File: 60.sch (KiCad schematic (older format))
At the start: 183 parts, among them IC1 ATXMEGA32A4U-A, J1 USB_mini_micro_B, K1 KEYSW, K10 KEYSW, K11 KEYSW, K12 KEYSW, K13 KEYSW, K14 KEYSW, K15 KEYSW, K16 KEYSW, K17 KEYSW, K18 KEYSW, K19 KEYSW, K2 KEYSW, K20 KEYSW, K21 KEYSW, K22 KEYSW, K23 KEYSW, K24 KEYSW, K25 KEYSW, K26 KEYSW, K27 KEYSW, K28 KEYSW, K29 KEYSW, K3 KEYSW, K30 KEYSW, K31 KEYSW, K32 KEYSW, K33 KEYSW, K34 KEYSW, K35 KEYSW, K36 KEYSW, K37 KEYSW, K38 KEYSW, K39 KEYSW, K4 KEYSW, K40 KEYSW, K41 KEYSW, K42 KEYSW, K43 KEYSW, K44 KEYSW, K45 KEYSW, K46 KEYSW, K47 KEYSW, K48 KEYSW, K49 KEYSW, K5 KEYSW, K50 KEYSW, K51 KEYSW, K52 KEYSW, K53 KEYSW, K54 KEYSW, K55 KEYSW, K56 KEYSW, K57 KEYSW, K58 KEYSW, K59 KEYSW, K6 KEYSW, K60 KEYSW, K61 KEYSW, K62 KEYSW, K63 KEYSW, K64 KEYSW, K65 KEYSW, K66 KEYSW, K67 KEYSW, K68 KEYSW, K69 KEYSW, K7 KEYSW, K70 KEYSW, K71 KEYSW, K72 KEYSW, K73 KEYSW, K74 KEYSW, K75 KEYSW, K76 KEYSW, K77 KEYSW, K78 KEYSW, K79 KEYSW, K8 KEYSW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

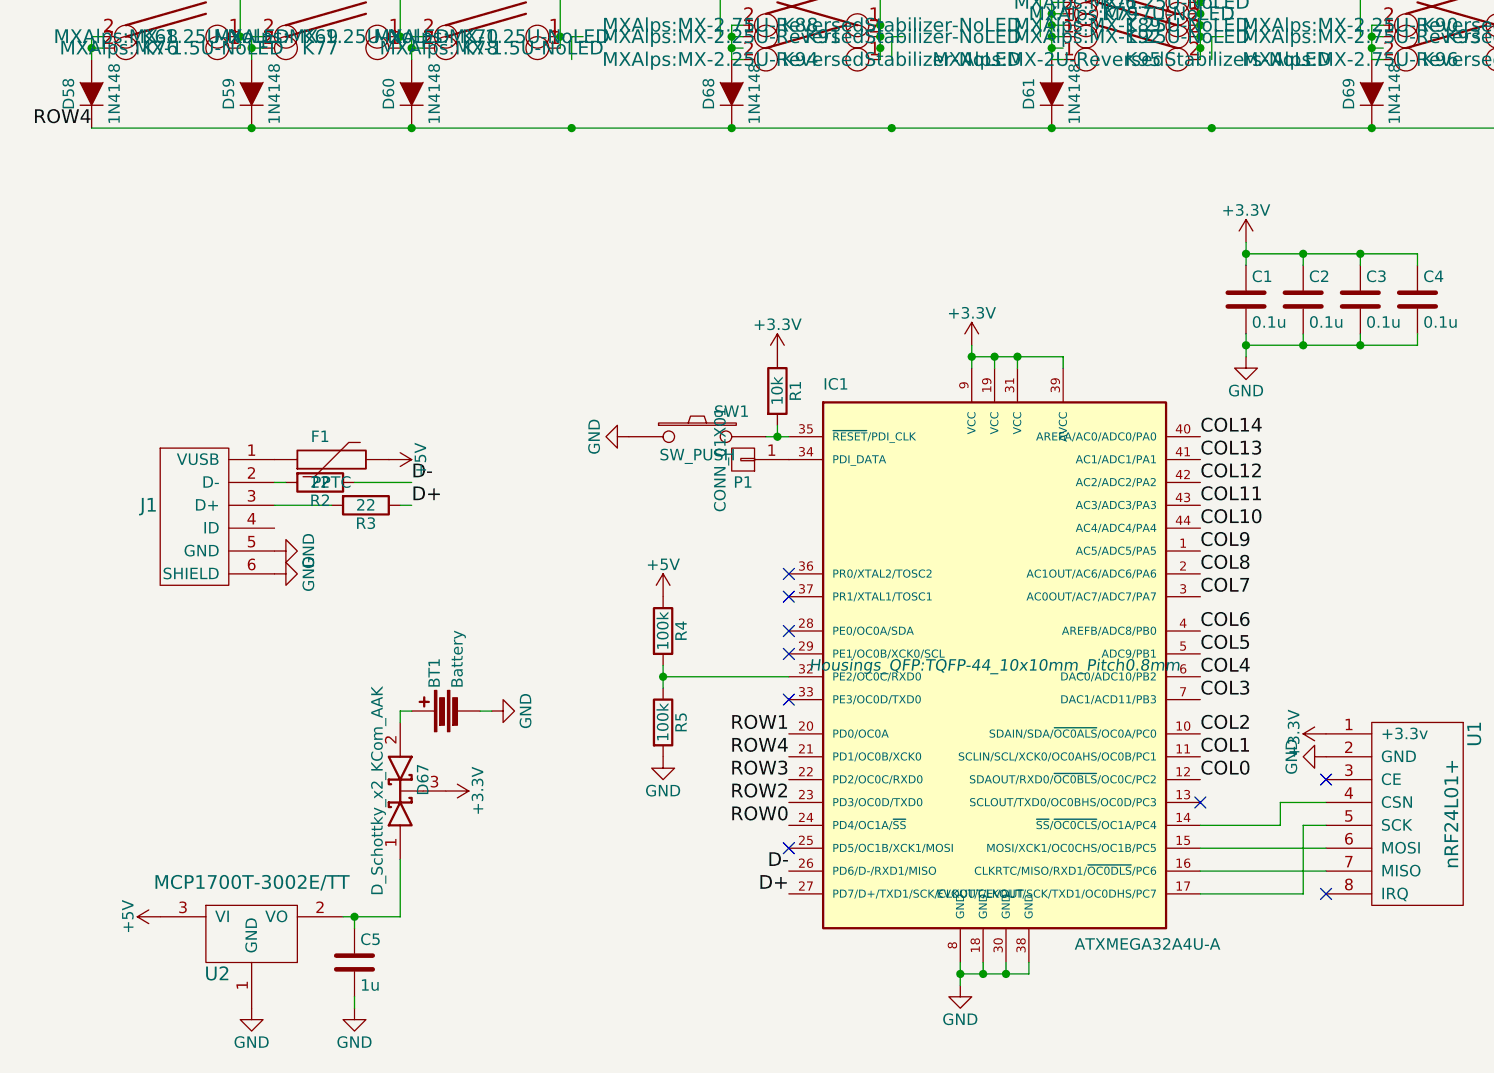
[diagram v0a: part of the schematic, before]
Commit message: Prototype 1
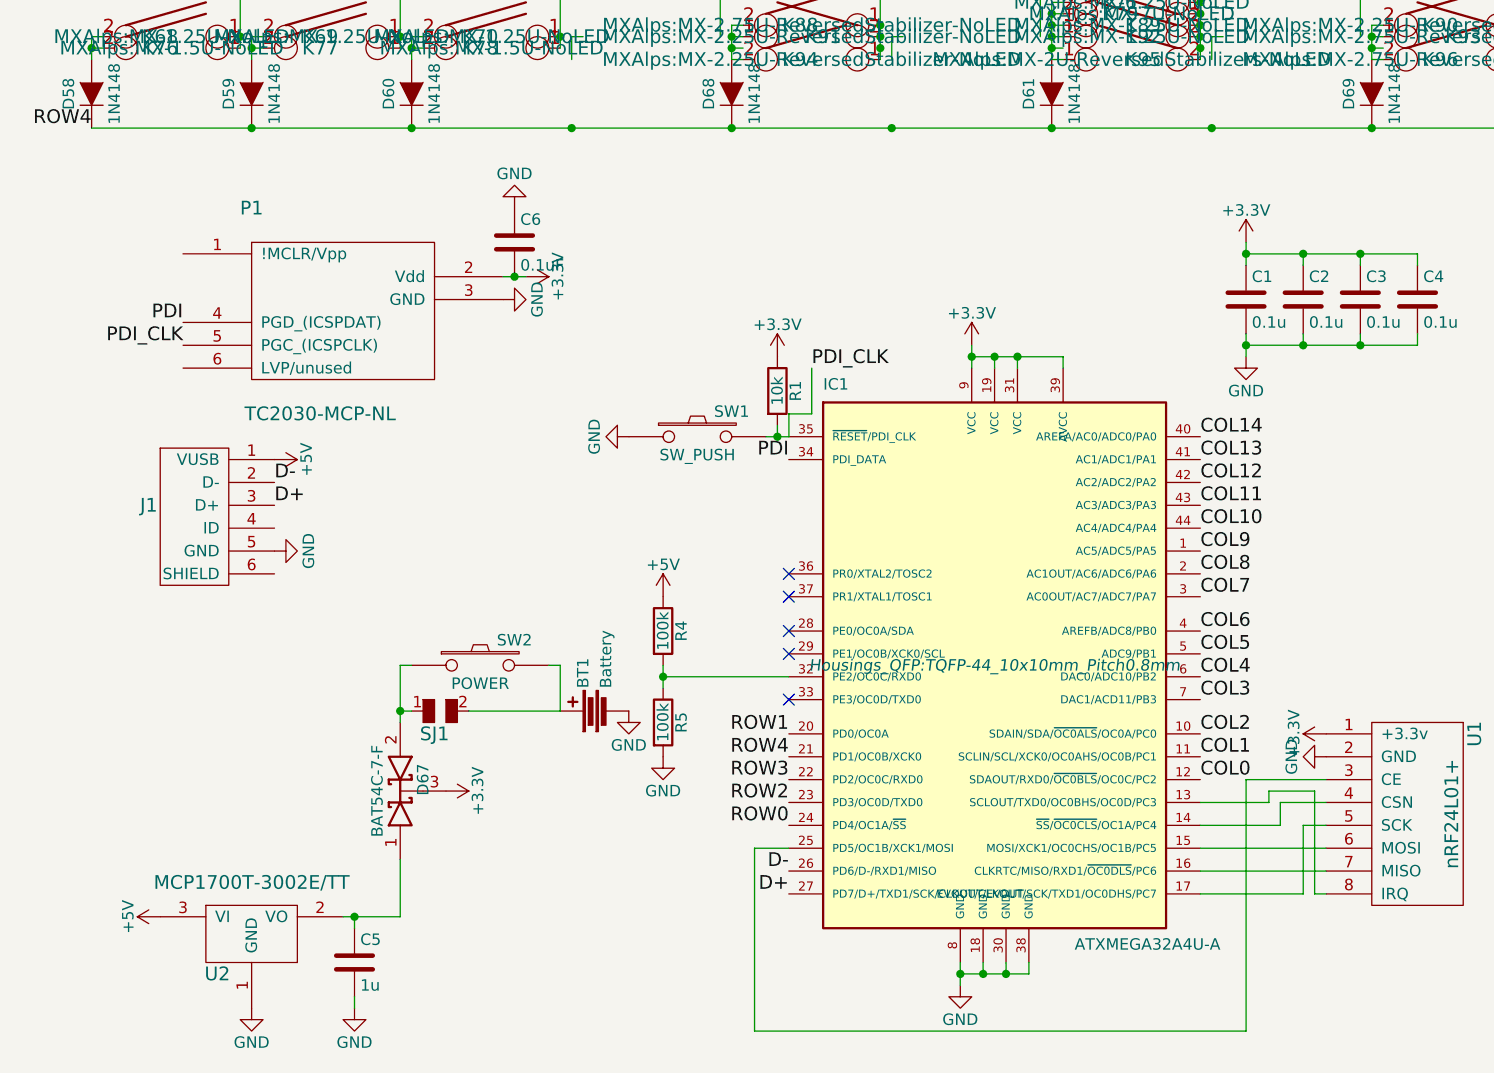
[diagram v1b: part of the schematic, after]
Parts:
- removed F1: PPTC, Fuse_Holders_and_Fuses:Fuse_SMD1206_HandSoldering, symbol PPTC
- removed P1: CONN_01X01, Connectors_TestPoints:Test_Point_Pad_d2.5mm, symbol CONN_01X01
- removed R2, R3: 22, Resistors_SMD:R_0805_HandSoldering, symbol R
- added C6: 0.1uF, Capacitors_SMD:C_0805_HandSoldering, symbol C
- added P1: TC2030-MCP-NL, Tag-Connect:TC2030-MCP-NL, symbol TC2030-MCP-NL
- added SJ1: SOLDER_JUMPER, keyboard_parts:SOLDER_JUMPER_2, symbol SOLDER_JUMPER
- added SW2: POWER, Pin_Headers:Pin_Header_Straight_1x02_Pitch2.54mm, symbol SW_PUSH
- BT1: footprint Battery_Holders:Keystone_1058_1x2032-CoinCell -> lib:CR2032_BK-913
- D67: value D_Schottky_x2_KCom_AAK -> BAT54C-7-F
- SW1: footprint Cartel:c&k_PTS645SH50SMTR92_LFS -> Buttons_Switches_SMD:SW_SPST_TL3342
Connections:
- net labels added: PDI, PDI_CLK
- wire segments 249 -> 262
- no-connect marks 9 -> 5
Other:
- moved on the sheet: BT1
